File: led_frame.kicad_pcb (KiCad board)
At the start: 2 copper layers, 150.7 x 231.5 mm, 102 parts, among them J1 Screw_Terminal_1x02, U1 Teensy-LC, U2 MIC_MAX4466, U3 StepDown_D24V50F5

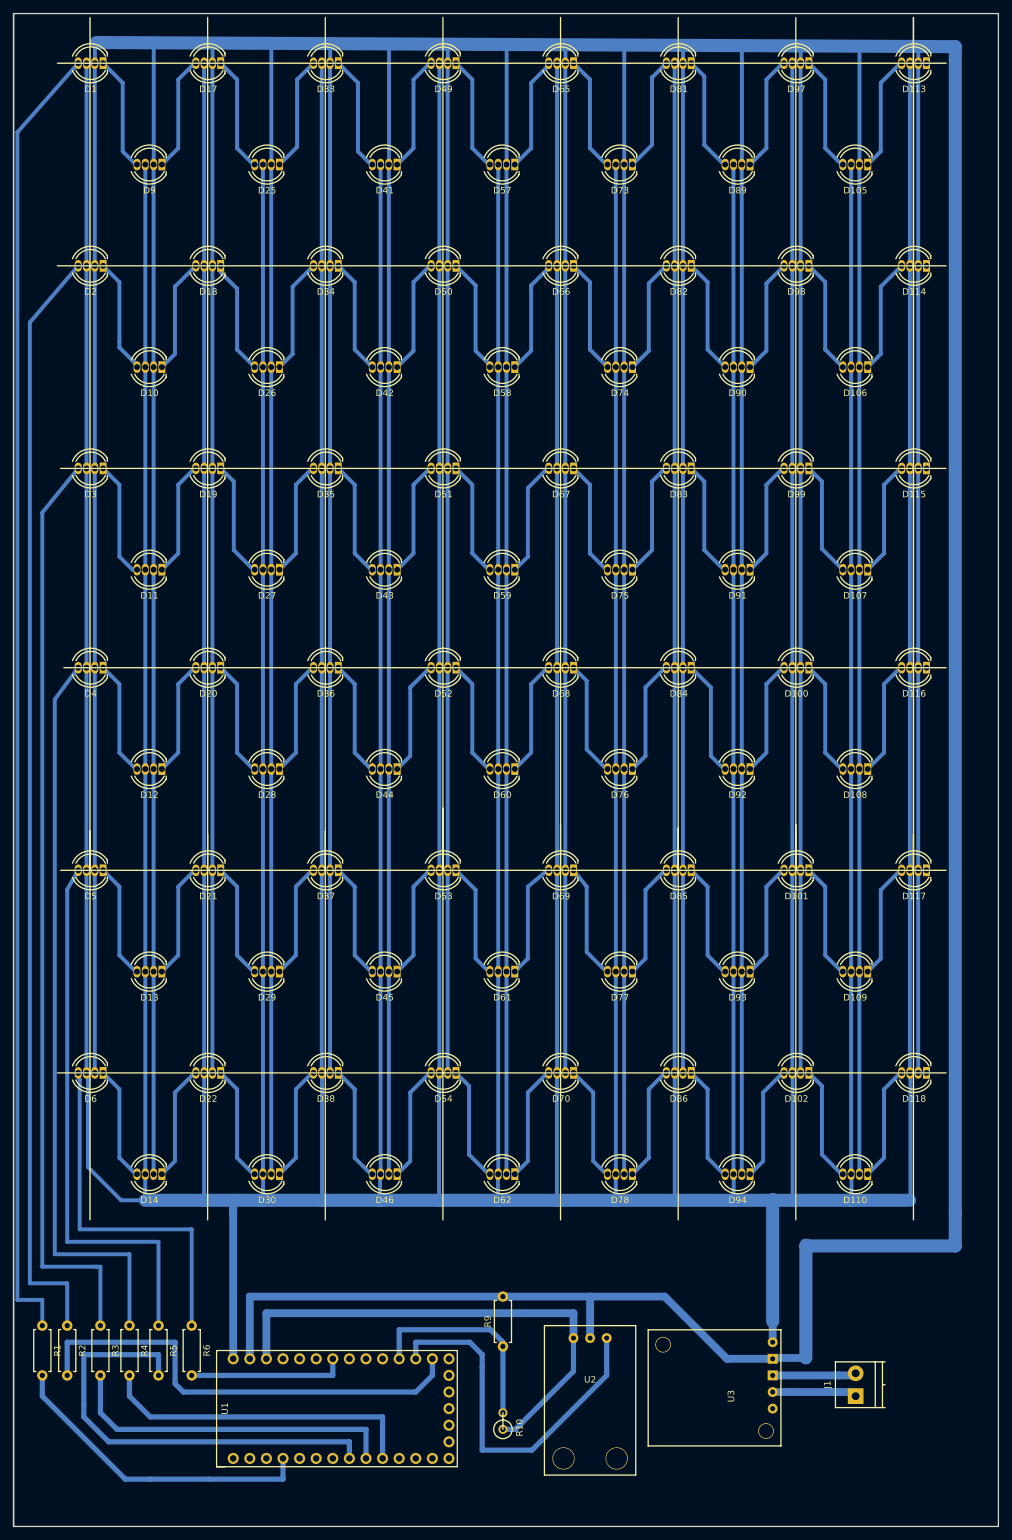
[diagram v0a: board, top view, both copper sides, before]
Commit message: fixing some connections
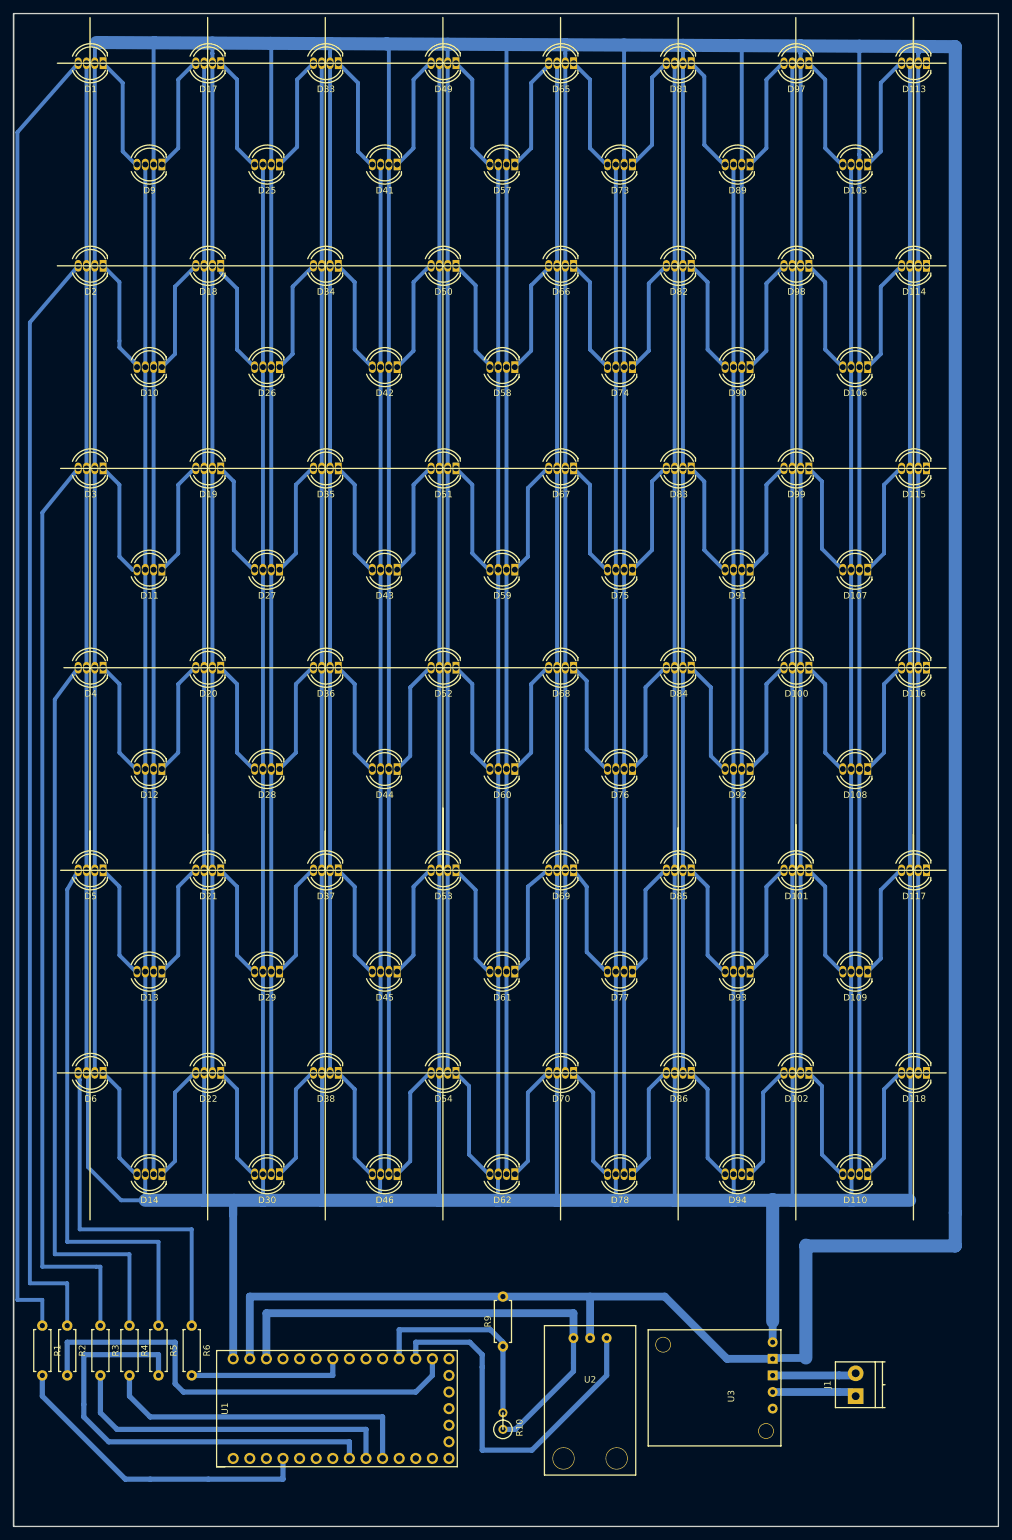
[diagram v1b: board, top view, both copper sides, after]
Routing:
- net Net-(D1-Pad2): track 3081.1 -> 2956.8 mm
